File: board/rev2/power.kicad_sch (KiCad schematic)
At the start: 21 parts, among them SW1 MS-22D28-G020, U1 TPD6S300A, U2 TPS62933

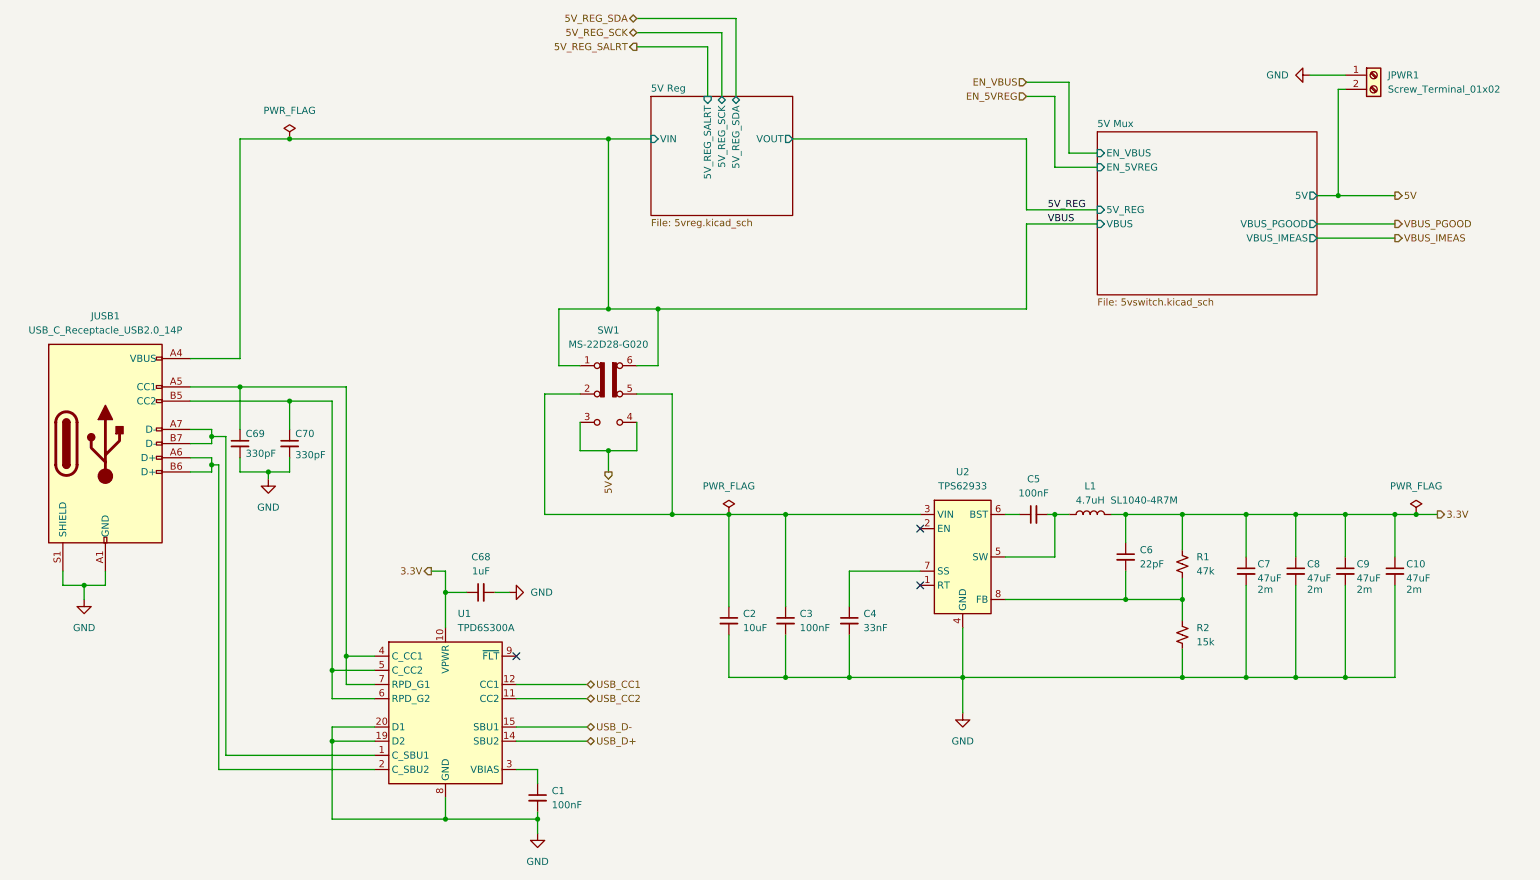
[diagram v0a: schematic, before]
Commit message: 3.3V LDO
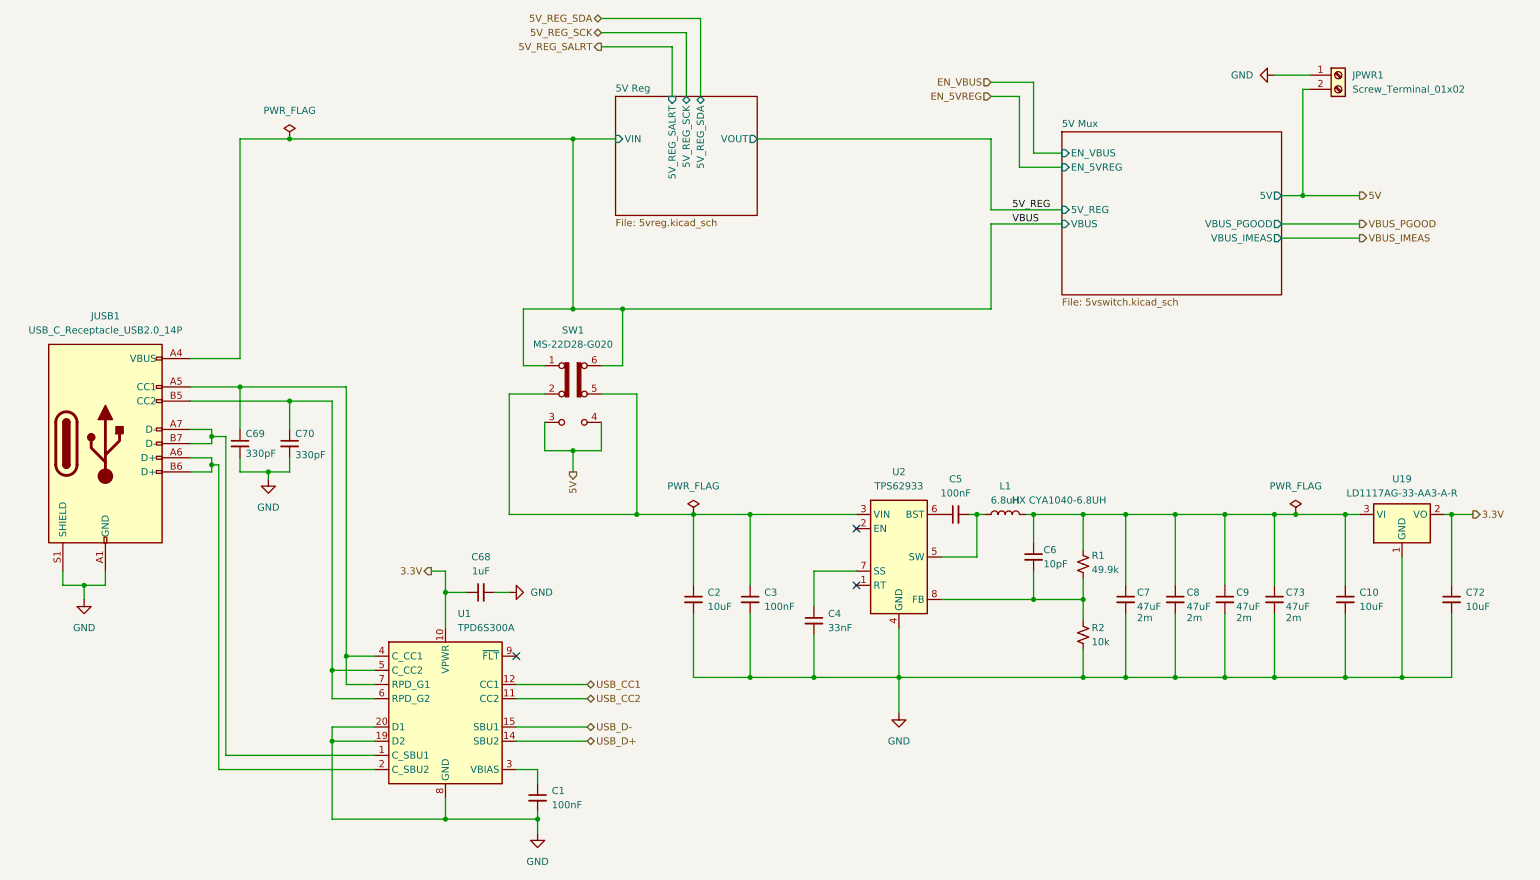
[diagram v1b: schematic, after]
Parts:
- added C72: 10uF, Capacitor_SMD:C_1210_3225Metric, symbol Device:C_Small
- added C73: 47uF, Capacitor_SMD:C_1206_3216Metric, symbol Device:C_Small
- added U19: LD1117AG-33-AA3-A-R, Package_TO_SOT_SMD:SOT-223-3_TabPin2, symbol Regulator_Linear:LD1117S33TR_SOT223
- C10: value 47uF -> 10uF; footprint Capacitor_SMD:C_1206_3216Metric -> Capacitor_SMD:C_1210_3225Metric; ESR 2m -> (none); LCSC C96123 -> C13585; Part CL31A476MPHNNNE -> CL31A106KBHNNNE
- C6: value 22pF -> 10pF; footprint Capacitor_SMD:C_0603_1608Metric -> Capacitor_SMD:C_0402_1005Metric; LCSC C1653 -> C32949; Part CL10C220JB8NNNC -> CL05C100JB5NNNC
- L1: value 4.7uH -> 6.8uH; footprint Inductor_SMD:L_TechFuse_SL1040 -> Inductor_SMD:L_Chilisin_BMRF00101040; LCSC C22463838 -> C7502775; Part SL1040-4R7M -> HX CYA1040-6.8UH
- R1: value 47k -> 49.9k; footprint Resistor_SMD:R_0805_2012Metric -> Resistor_SMD:R_0603_1608Metric; LCSC C17713 -> C23184; Part 0805W8F4702T5E -> 0603WAF4992T5E
- R2: value 15k -> 10k; footprint Resistor_SMD:R_0805_2012Metric -> Resistor_SMD:R_0402_1005Metric; LCSC C17475 -> C25744; Part 0805W8F1502T5E -> 0402WGF1002TCE
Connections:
- net 3.3V: now also C72.1, U19.2 (VO); no longer C10.1, C6.1, C7.1, C8.1, C9.1, L1.2, R1.1
- net GND: now also C72.2, C73.2, U19.1 (GND)
- new net: C10.1, C6.1, C7.1, C73.1, C8.1, C9.1, L1.2, R1.1, U19.3 (VI)
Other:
- moved on the sheet: C2, C3, C4, C5, C6, C7, C8, C9, JPWR1, L1, SW1, U2
